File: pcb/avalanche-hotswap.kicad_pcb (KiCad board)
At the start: 2 copper layers, 179.7 x 122.7 mm, 139 parts, among them J1 TRRS, J2 OLED, P1 i2c_pin, P2 i2c_pin, P3 battery+, P4 battery-, SW0 SW_Push, SW1 SW_Push, SW10 SW_Push, SW11 SW_Push, SW12 SW_Push, SW13 SW_Push, SW14 SW_Push, SW15 SW_Push, SW16 SW_Push, SW17 SW_Push, SW18 SW_Push, SW19 SW_Push, SW2 SW_Push, SW20 SW_Push, SW21 SW_Push, SW22 SW_Push, SW23 SW_Push, SW24 SW_Push, SW25 SW_Push, SW26 SW_Push, SW27 SW_Push, SW28 SW_Push, SW29 SW_Push, SW3 SW_Push, SW30 SW_Push, SW31 SW_Push, SW32 SW_Push, SW33 SW_DPDT_x2, SW34 SW_DPDT_x2, SW4 SW_Push, SW5 SW_Push, SW6 SW_Push, SW7 SW_Push, SW8 SW_Push, SW9 SW_Push, U1 ProMicro

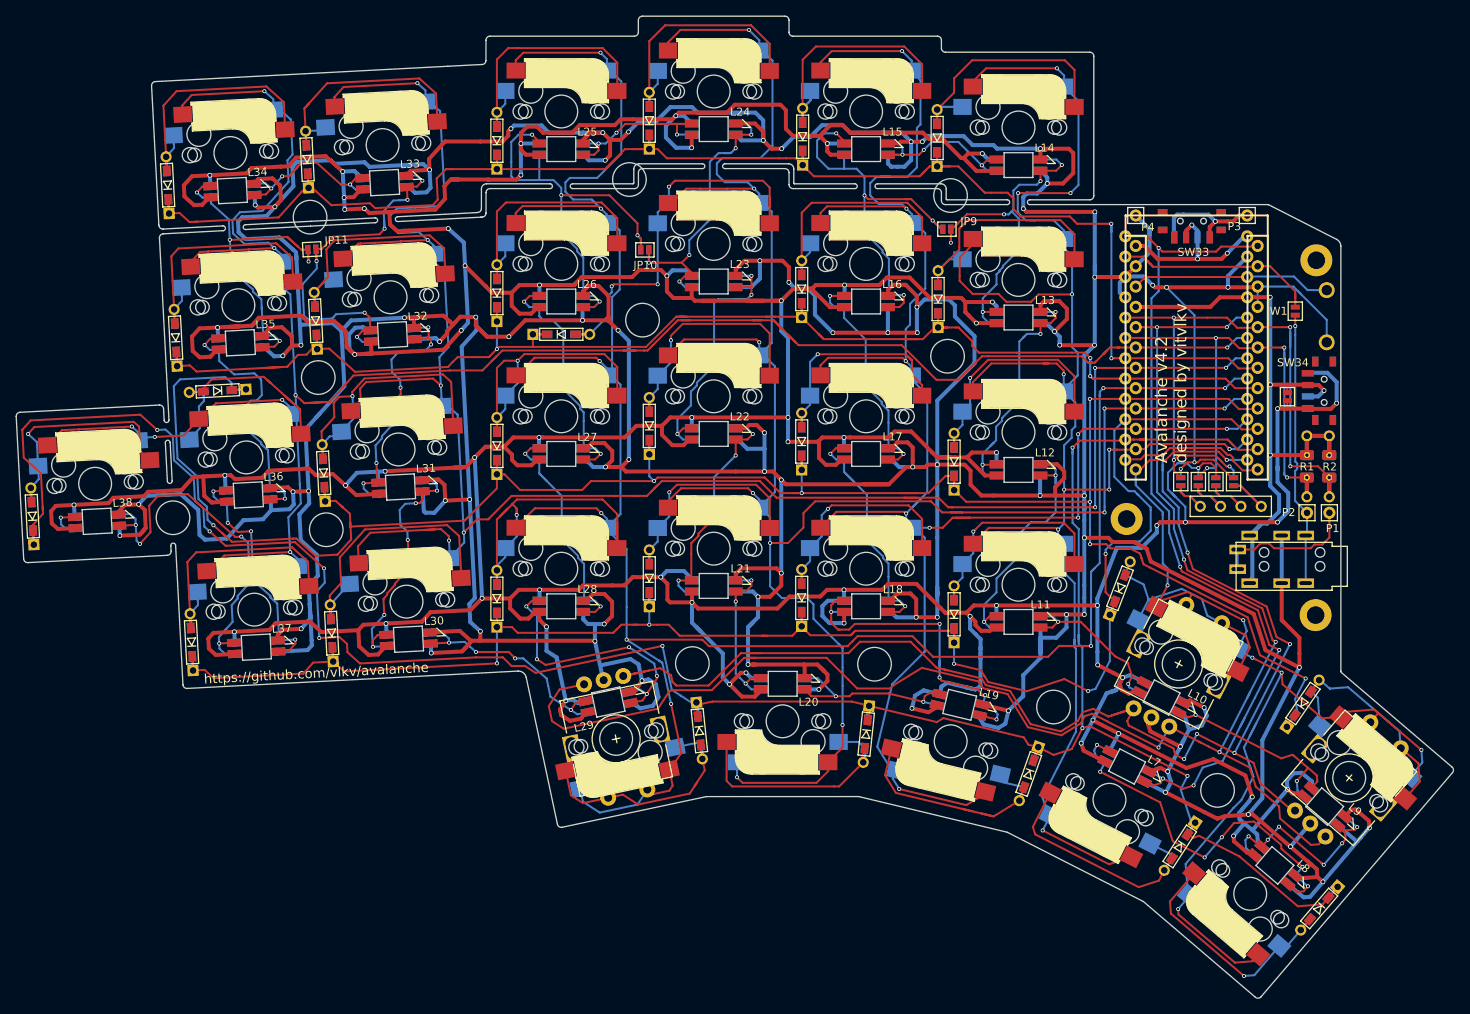
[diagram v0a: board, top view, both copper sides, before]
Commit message: Checkpoint commit with merge from upstream.
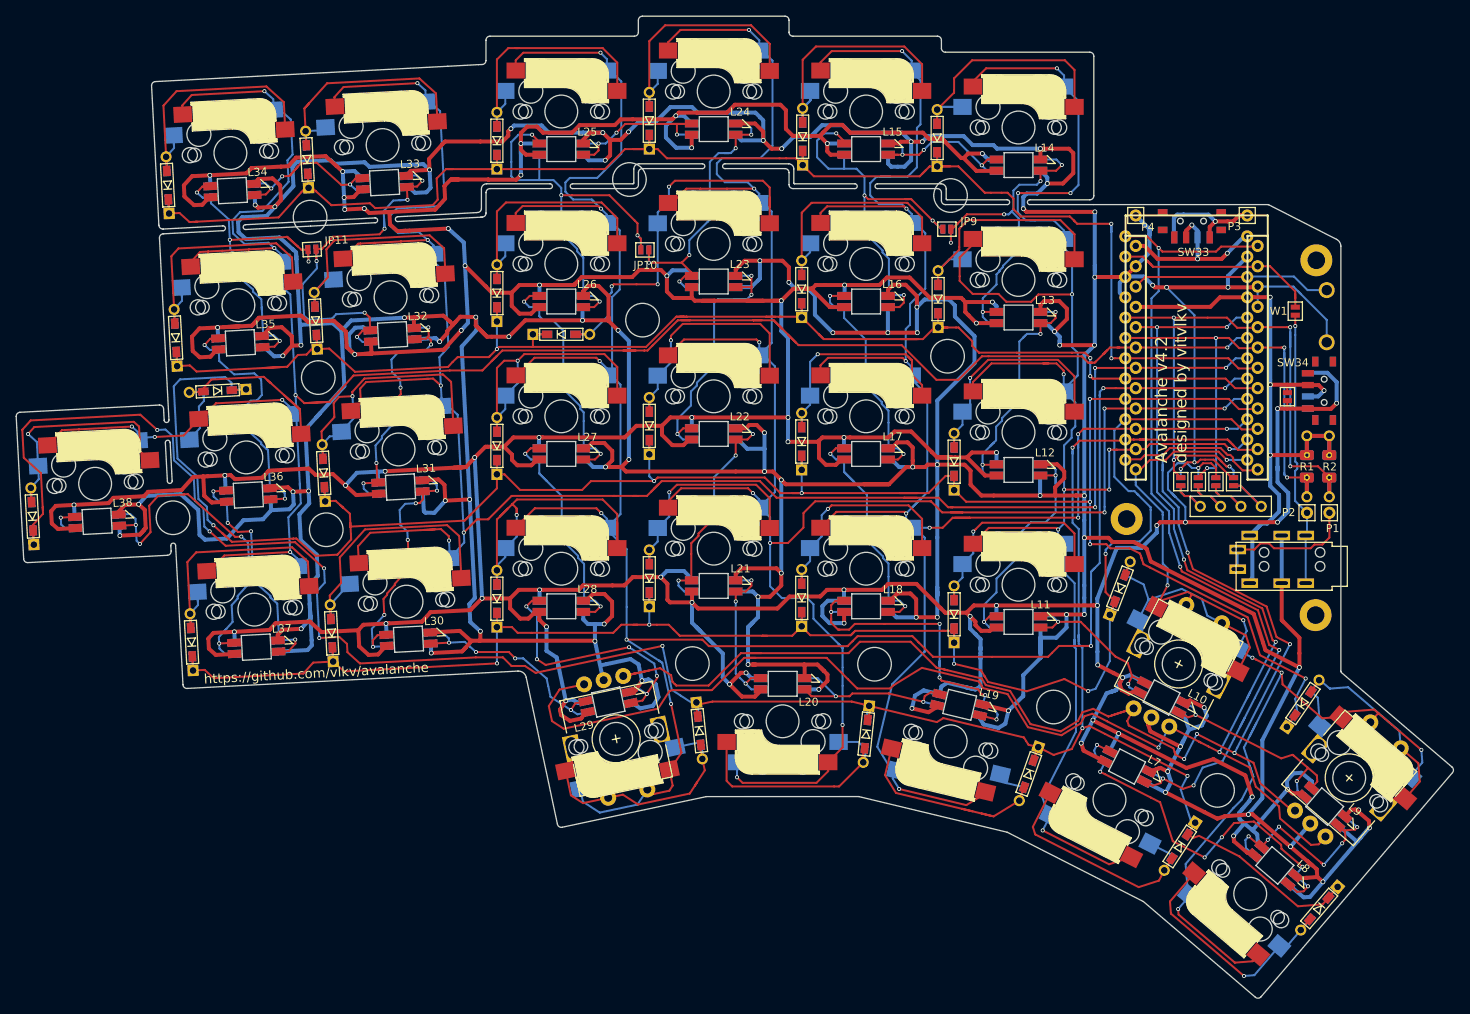
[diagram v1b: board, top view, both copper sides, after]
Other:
- outline, holes or cut-outs redrawn
- net class Default removed
